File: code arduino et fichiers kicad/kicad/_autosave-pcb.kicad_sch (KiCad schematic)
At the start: 34 parts, among them J1 Screw_Terminal_01x04, J2 Screw_Terminal_01x04, J3 Screw_Terminal_01x02, U1 LMC6482, U2 LMC6482, U3 LMC6482

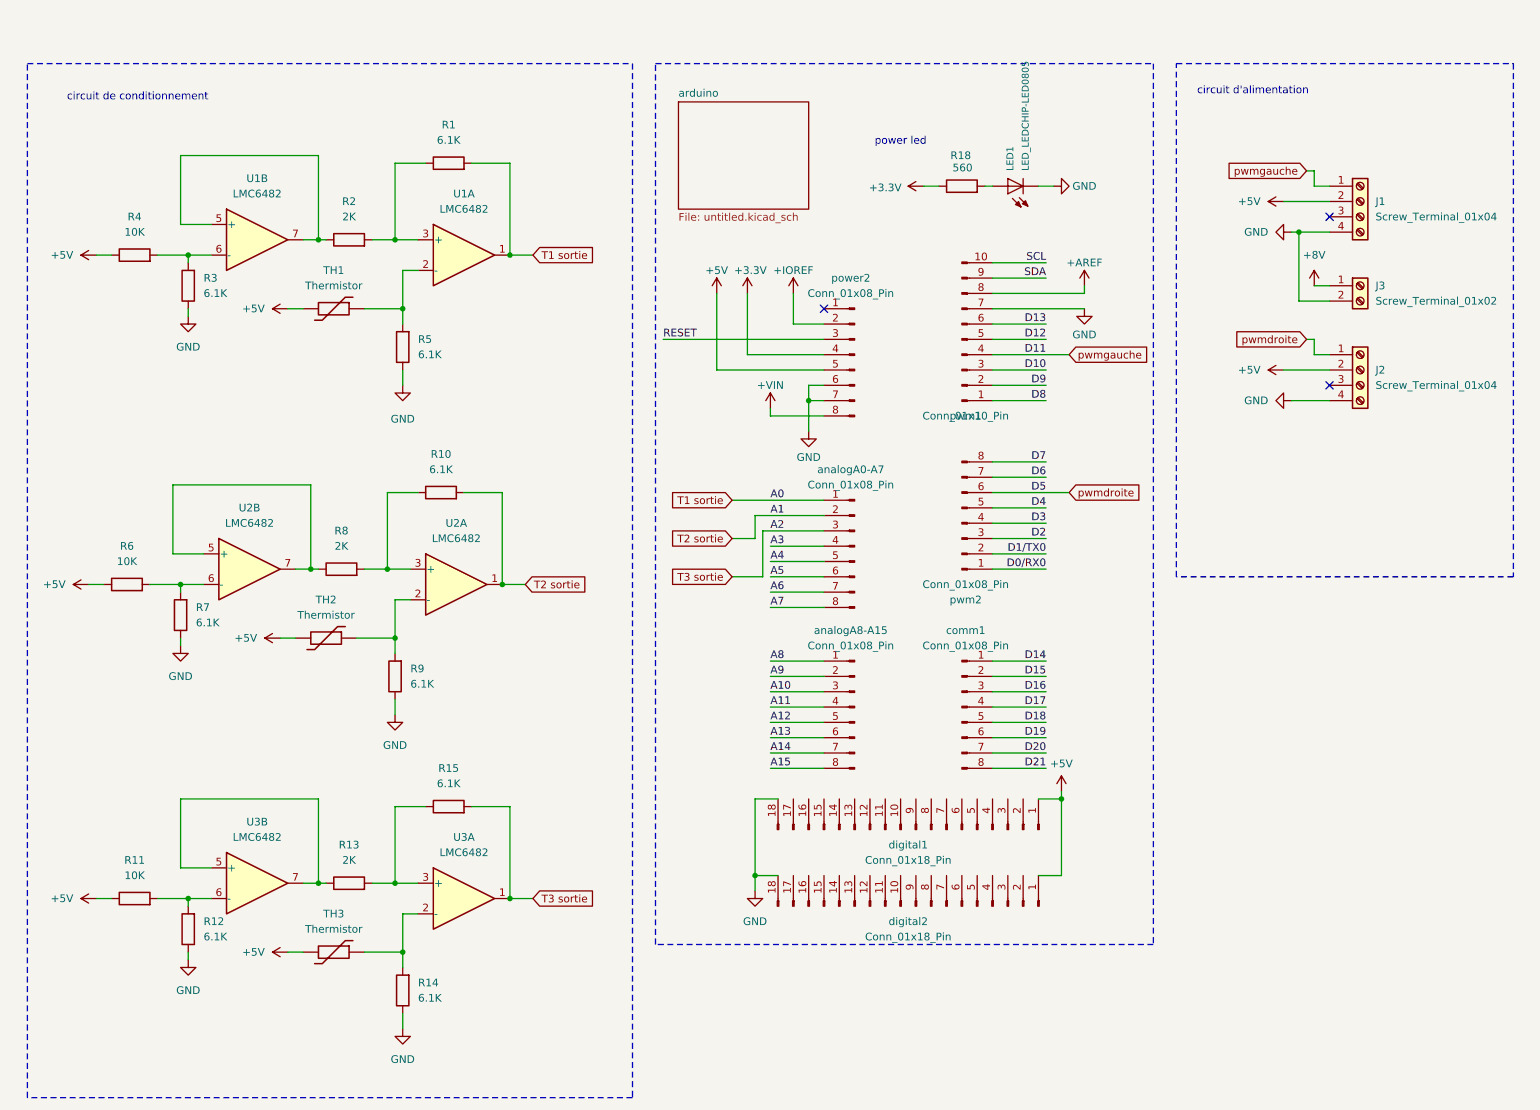
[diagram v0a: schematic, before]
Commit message: ksjkasjdh
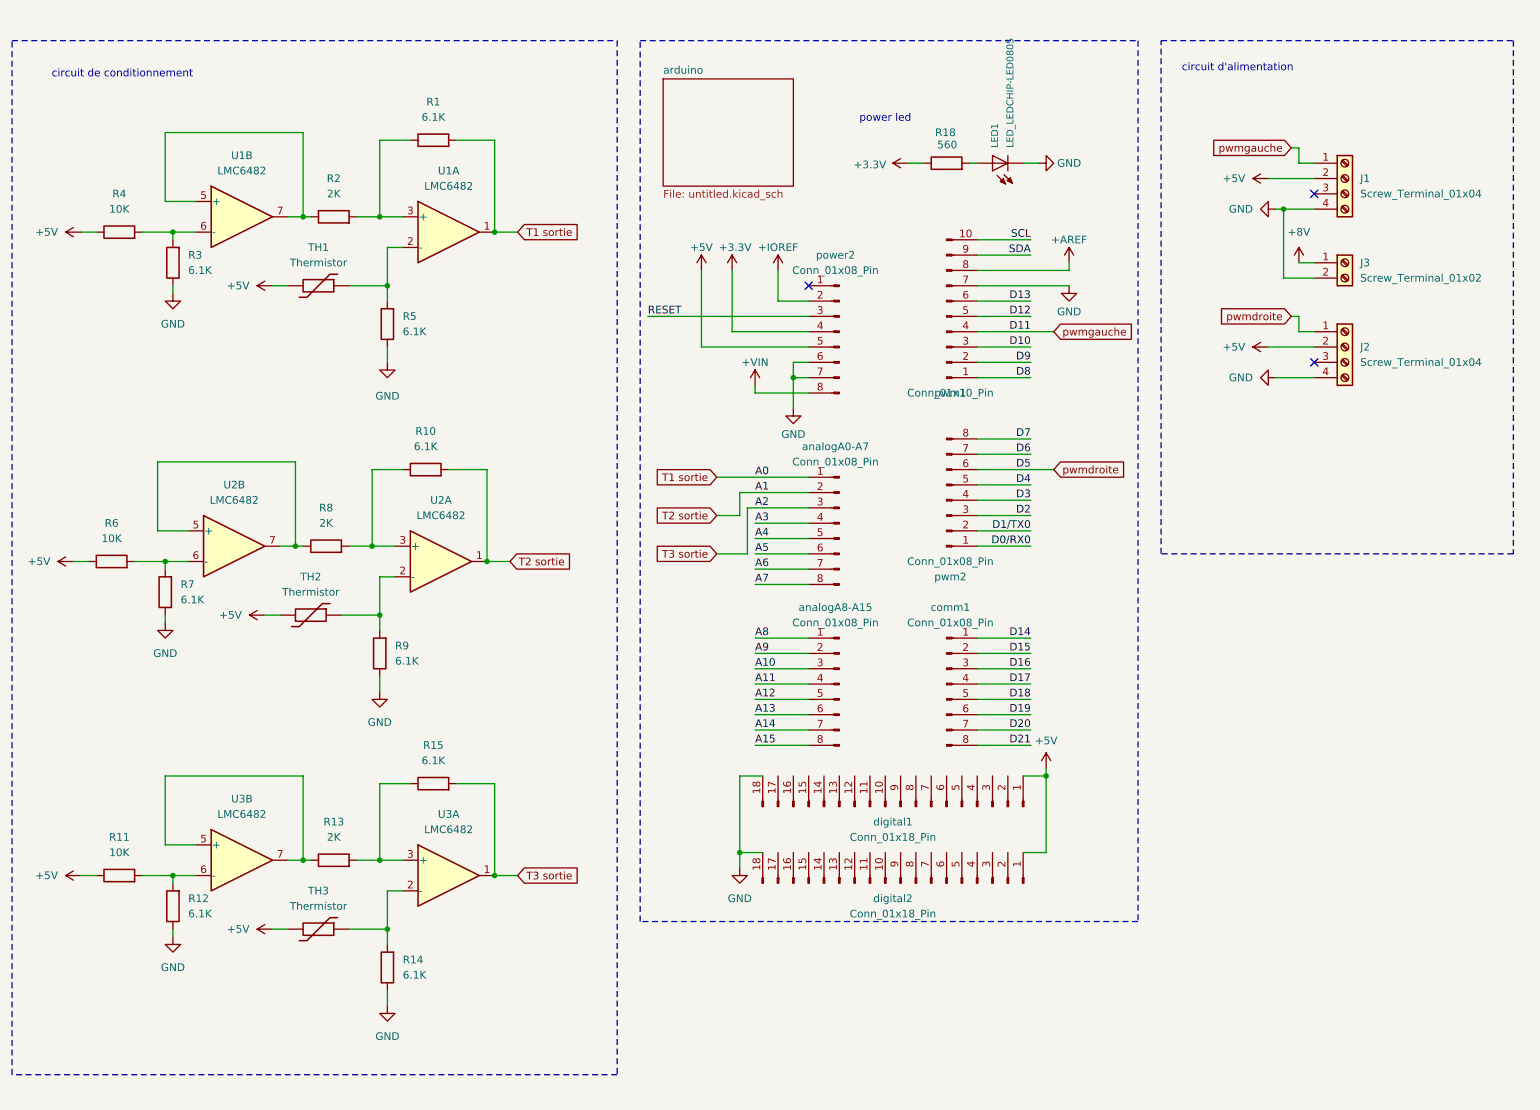
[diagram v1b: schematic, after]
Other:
- moved on the sheet: J1, J2, J3, LED1, R1, R10, R11, R12, R13, R14, R15, R18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
